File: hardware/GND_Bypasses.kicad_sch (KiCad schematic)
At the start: 12 parts, among them Q1 NPN

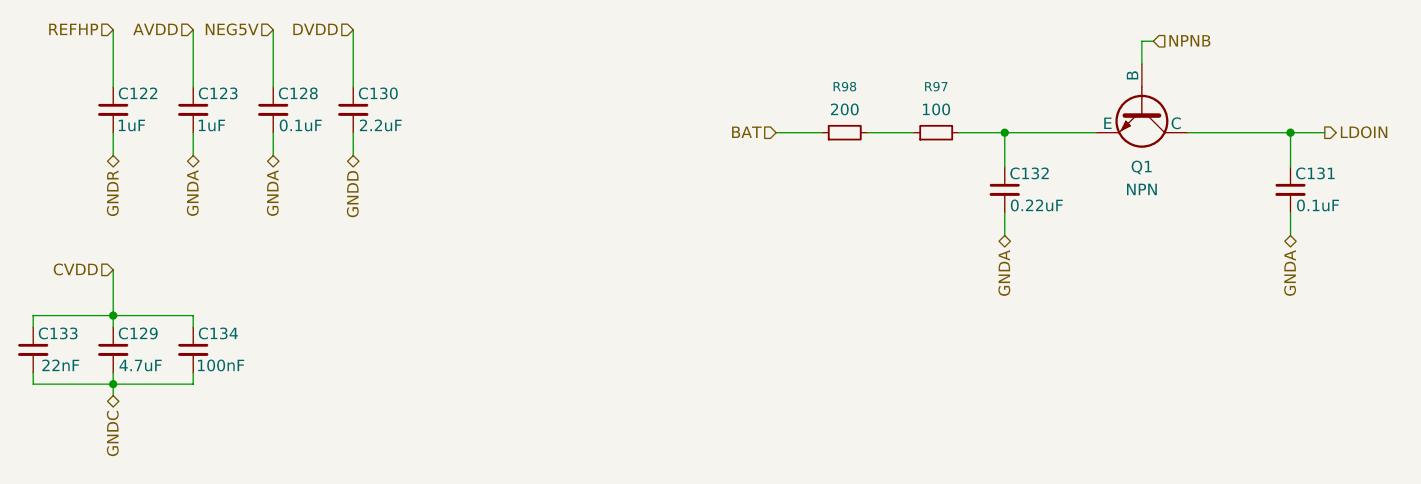
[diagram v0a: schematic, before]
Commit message: updated sheets and 1st review changes
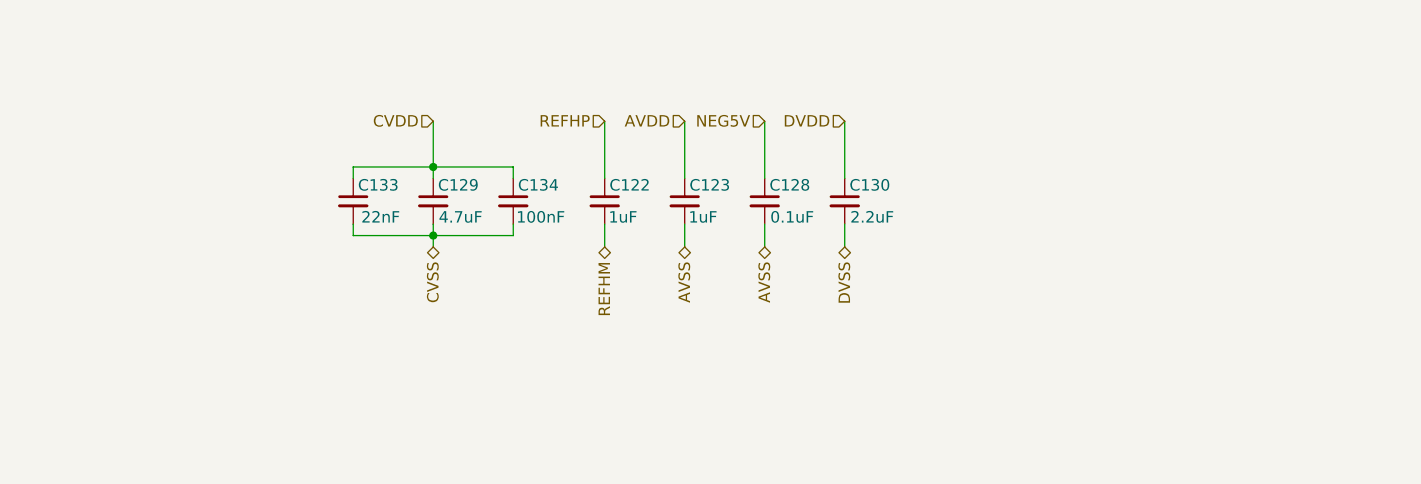
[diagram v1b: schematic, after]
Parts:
- removed C131: 0.1uF, symbol Device:C_Small
- removed C132: 0.22uF, symbol Device:C_Small
- removed Q1: NPN, symbol Simulation_SPICE:NPN
- removed R97: 100, symbol Device:R_Small
- removed R98: 200, symbol Device:R_Small
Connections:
- net GNDA renamed AVSS
- net GNDC renamed CVSS
- net GNDD renamed DVSS
- net GNDR renamed REFHM
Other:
- moved on the sheet: C122, C123, C128, C129, C130, C133, C134
